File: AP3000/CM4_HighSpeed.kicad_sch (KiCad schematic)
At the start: 5 parts, among them J4 Conn_01x22_Female, J5 Conn_01x22_Female

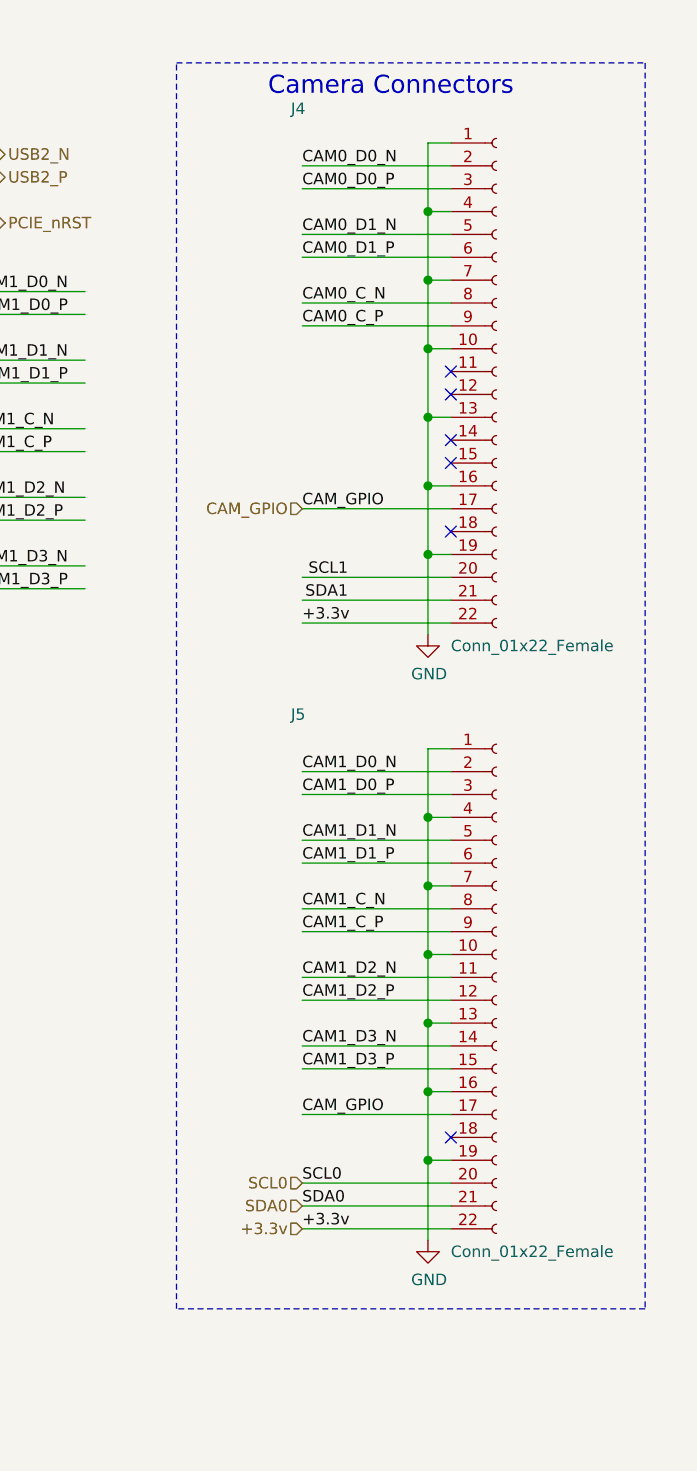
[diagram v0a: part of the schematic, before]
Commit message: Route more
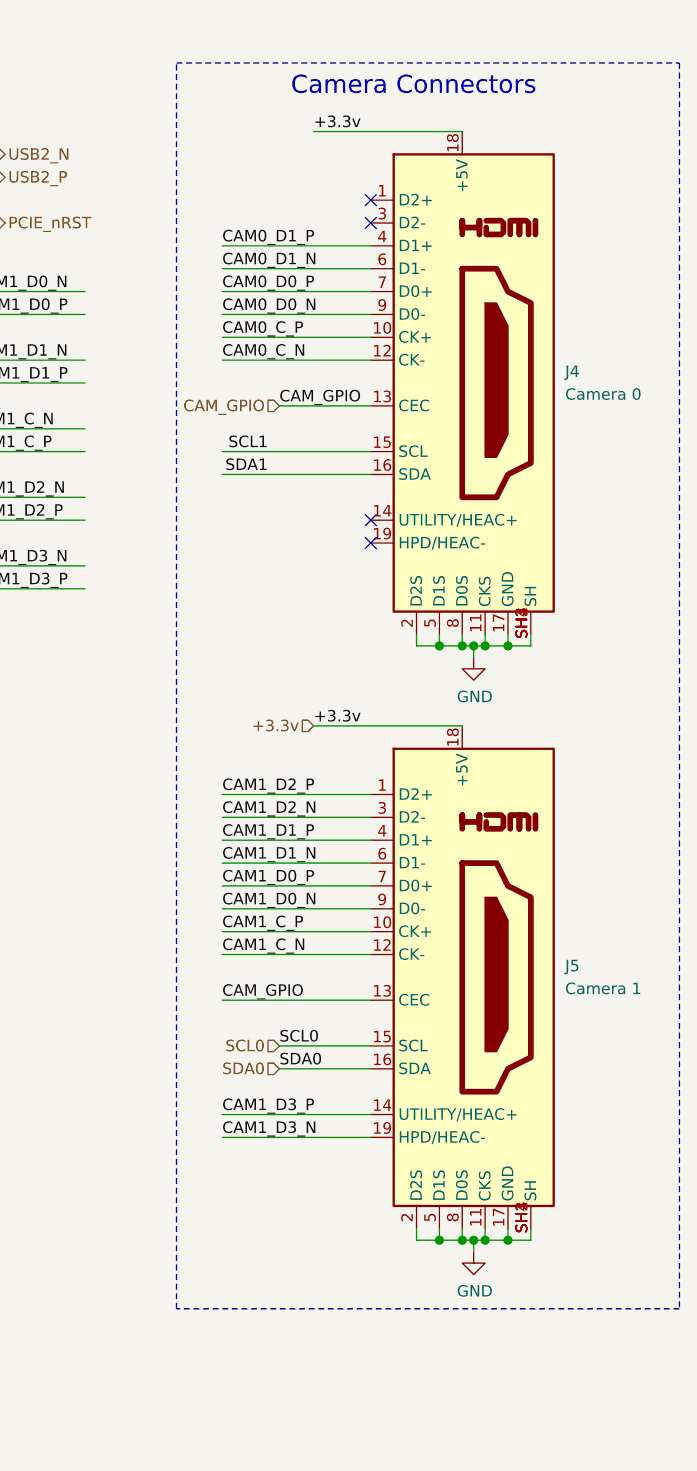
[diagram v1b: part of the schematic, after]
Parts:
- removed J4, J5: Conn_01x22_Female, Connector_FFC-FPC:Hirose_FH12-22S-0.5SH_1x22-1MP_P0.50mm_Horizontal, symbol Connector:Conn_01x22_Female
- added J4: Camera 0, AP3000:EDAC 690-019-298-412, symbol AP3000:HDMI_A_1.4
- added J5: Camera 1, AP3000:EDAC 690-019-298-412, symbol AP3000:HDMI_A_1.4
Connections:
- net +3.3v: now also J4.18 (+5V), J5.18 (+5V)
- net CAM0_C_N: now also J4.12 (CK-)
- net CAM0_C_P: now also J4.10 (CK+)
- net CAM0_D0_N: now also J4.9 (D0-)
- net CAM0_D0_P: now also J4.7 (D0+)
- net CAM0_D1_N: now also J4.6 (D1-)
- net CAM0_D1_P: now also J4.4 (D1+)
- net CAM1_C_N: now also J5.12 (CK-)
- net CAM1_C_P: now also J5.10 (CK+)
- net CAM1_D0_N: now also J5.9 (D0-)
- net CAM1_D0_P: now also J5.7 (D0+)
- net CAM1_D1_N: now also J5.6 (D1-)
- net CAM1_D1_P: now also J5.4 (D1+)
- net CAM1_D2_N: now also J5.3 (D2-)
- net CAM1_D2_P: now also J5.1 (D2+)
- net CAM1_D3_N: now also J5.19 (HPD/HEAC-)
- net CAM1_D3_P: now also J5.14 (UTILITY/HEAC+)
- net CAM_GPIO: now also J4.13 (CEC), J5.13 (CEC)
- net GND: now also J4.11 (CKS), J4.17 (GND), J4.2 (D2S), J4.5 (D1S), J4.8 (D0S), J4.SH1 (SH), J4.SH2 (SH), J4.SH3 (SH), J4.SH4 (SH), J5.11 (CKS), J5.17 (GND), J5.2 (D2S), J5.5 (D1S), J5.8 (D0S), J5.SH1 (SH), J5.SH2 (SH), J5.SH3 (SH), J5.SH4 (SH)
- net ID_SC: now also J4.15 (SCL)
- net ID_SD: now also J4.16 (SDA)
- net SCL0: now also J5.15 (SCL)
- net SDA0: now also J5.16 (SDA)
- no-connect marks 50 -> 48
